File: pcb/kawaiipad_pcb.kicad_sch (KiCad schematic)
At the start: 28 parts, among them SW1 SW_Push_45deg, SW2 SW_Push_45deg, SW3 SW_Push_45deg, SW4 SW_Push_45deg, SW5 SW_Push_45deg, SW6 SW_Push_45deg, SW7 SW_Push_45deg, SW8 SW_Push_45deg, SW9 SW_Push_45deg, U1 XIAO-RP2040-DIP

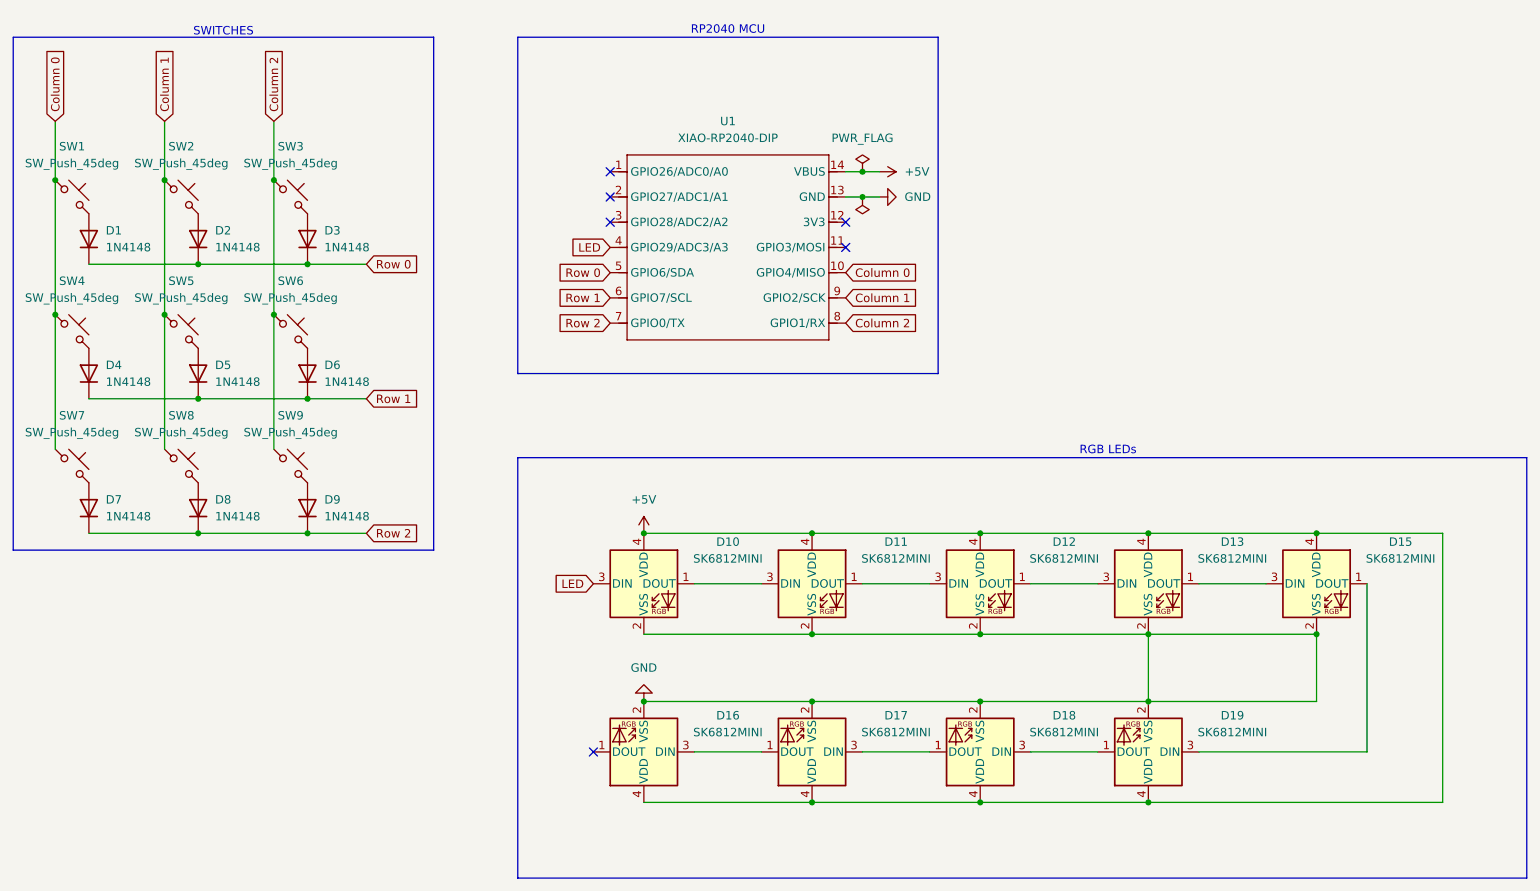
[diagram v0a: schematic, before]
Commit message: finish PCB wiring
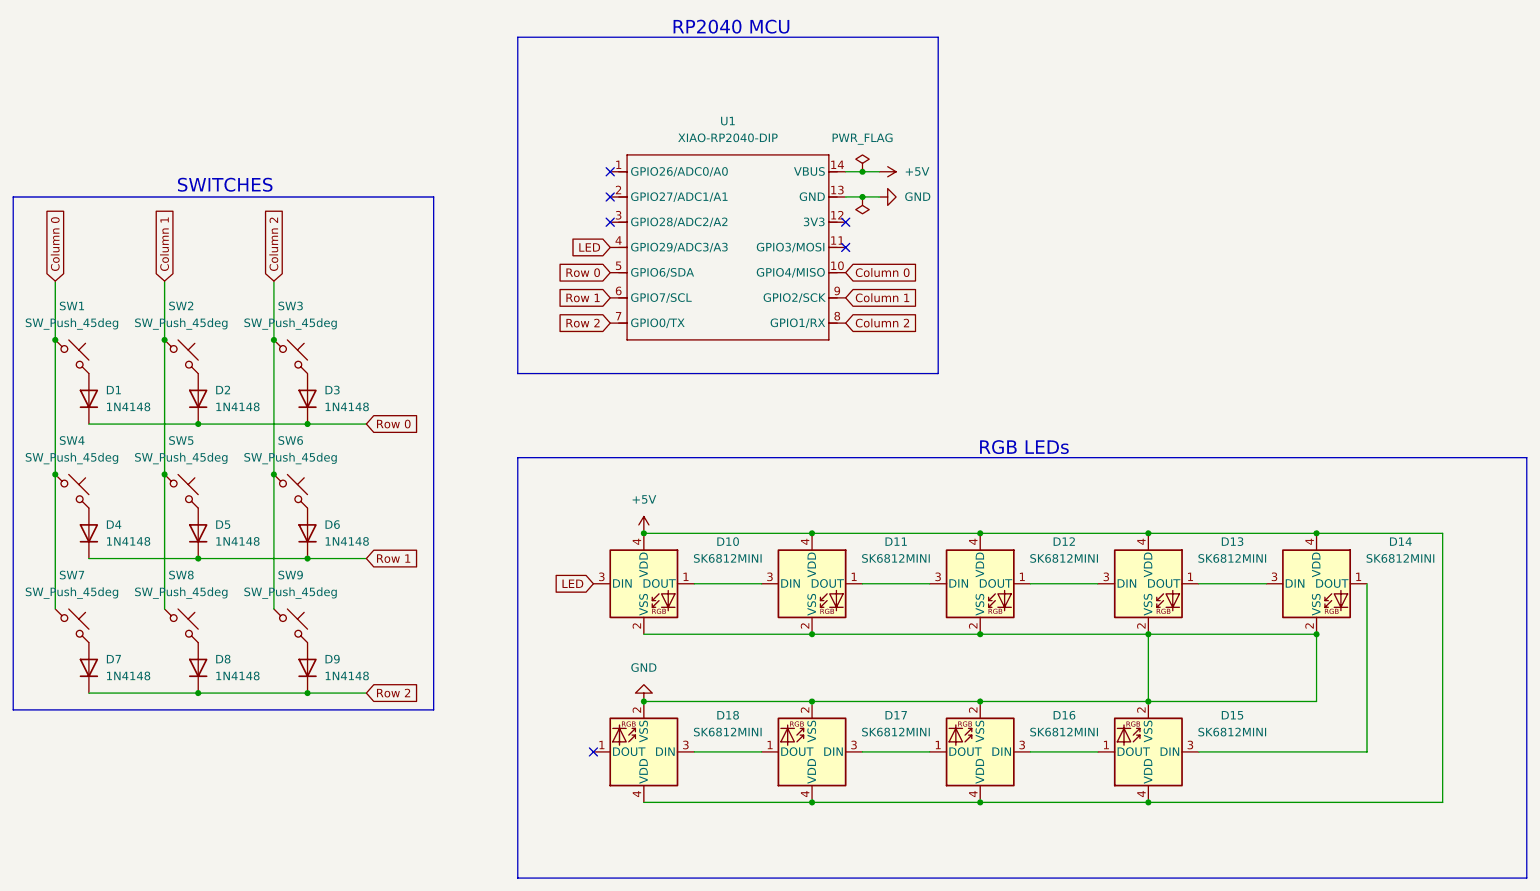
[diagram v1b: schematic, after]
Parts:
- removed D19: SK6812MINI, LED_SMD:LED_SK6812MINI_PLCC4_3.5x3.5mm_P1.75mm, symbol LED:SK6812MINI
- added D14: SK6812MINI, LED_SMD:LED_SK6812MINI_PLCC4_3.5x3.5mm_P1.75mm, symbol LED:SK6812MINI
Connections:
- net +5V: now also D14.4 (VDD)
- net GND: now also D14.2 (VSS)
- net at D16.1 (DOUT): now also D17.3 (DIN)
- net at D17.1 (DOUT): now also D18.3 (DIN); no longer D16.3 (DIN)
- net at D15.3 (DIN): now also D14.1 (DOUT); no longer D13.1 (DOUT)
- net at D15.1 (DOUT): now also D16.3 (DIN)
- net at D18.1 (DOUT): no longer D17.3 (DIN)
- new net: D13.1 (DOUT), D14.3 (DIN)
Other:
- moved on the sheet: D1, D2, D3, D4, D5, D6, D7, D8, D9, SW1, SW2, SW3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
